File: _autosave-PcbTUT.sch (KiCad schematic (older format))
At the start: 14 parts, among them SW1 SW_Push, U1 ATmega32U4-AU, Y1 16Mhz

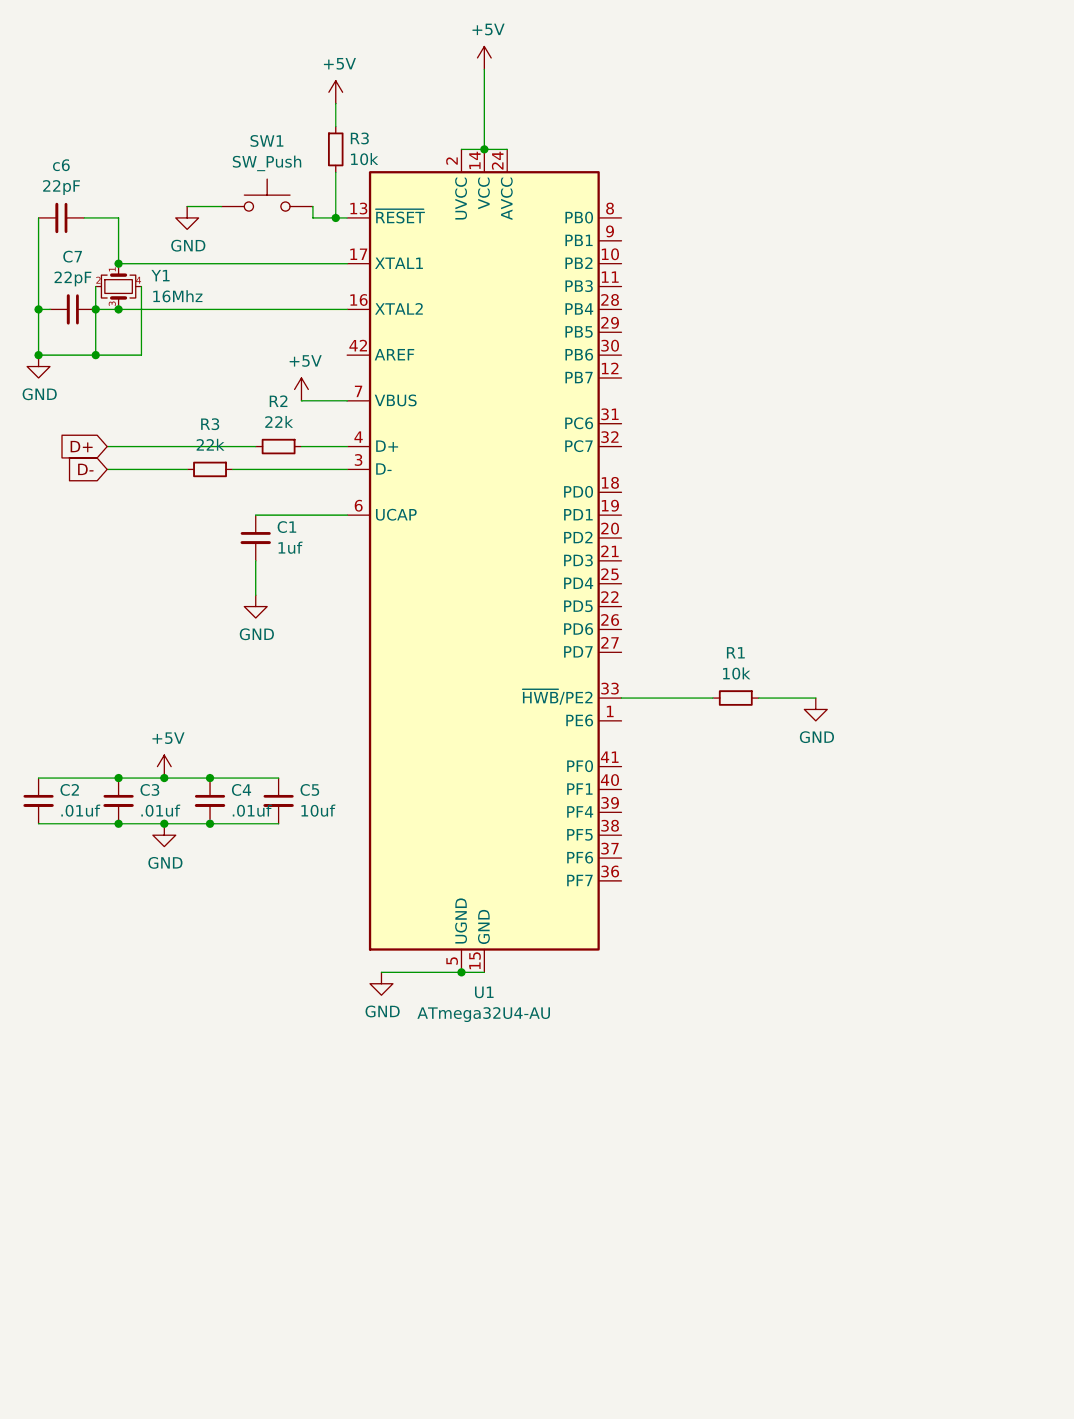
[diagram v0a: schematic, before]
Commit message: up to step 7
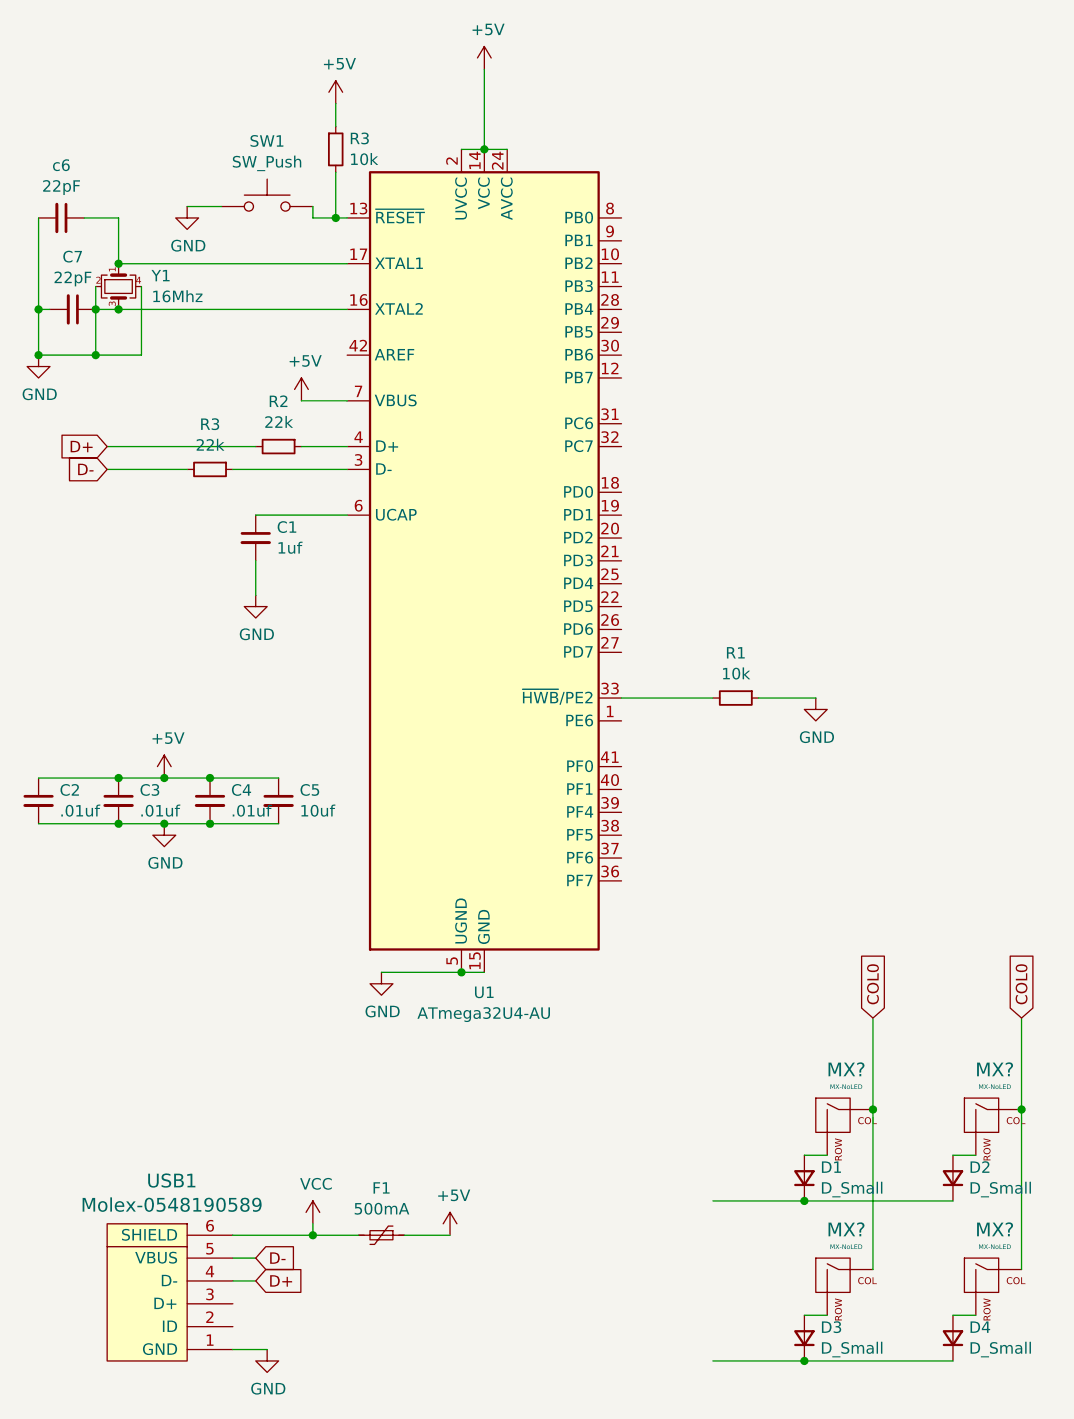
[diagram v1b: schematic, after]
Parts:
- added D1, D2, D3, D4: D_Small, symbol Device:D_Small
- added F1: 500mA, symbol Device:Polyfuse_Small
- added MX? (x4): MX-NoLED, symbol MX_Alps_Hybrid:MX-NoLED
- added USB1: Molex-0548190589, symbol random-keyboard-parts:Molex-0548190589
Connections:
- net labels added: COL0, VCC
- wire segments 41 -> 60
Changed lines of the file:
@@
 Text GLabel 850  2800 0    50   Input ~ 0
 D-
+$Comp
+L random-keyboard-parts:Molex-0548190589 USB1
+U 1 1 5EFB8536
+P 1100 6450
+F 0 "USB1" V 1637 6417 60  0000 C CNN
+F 1 "Molex-0548190589" V 1531 6417 60  0000 C CNN
+F 2 "" H 1100 6450 60  0001 C CNN
+F 3 "" H 1100 6450 60  0001 C CNN
+	1    1100 6450
+	0    -1   -1   0
+$EndComp
+$Comp
+L power:GND #PWR?
+U 1 1 5EFBB31B
+P 1550 6650
+F 0 "#PWR?" H 1550 6400 50  0001 C CNN
+F 1 "GND" H 1555 6477 50  0000 C CNN
+F 2 "" H 1550 6650 50  0001 C CNN
+F 3 "" H 1550 6650 50  0001 C CNN
+	1    1550 6650
+	1    0    0    -1
+$EndComp
+Wire Wire Line
+	1400 6650 1550 6650
+$Comp
+L power:+5V #PWR?
+U 1 1 5EFBCC7A
+P 2350 6150
+F 0 "#PWR?" H 2350 6000 50  0001 C CNN
+F 1 "+5V" H 2365 6323 50  0000 C CNN
+F 2 "" H 2350 6150 50  0001 C CNN
+F 3 "" H 2350 6150 50  0001 C CNN
+	1    2350 6150
+	1    0    0    -1
+$EndComp
+$Comp
+L Device:Polyfuse_Small F1
+U 1 1 5EFBDF67
+P 2050 6150
+F 0 "F1" V 1845 6150 50  0000 C CNN
+F 1 "500mA" V 1936 6150 50  0000 C CNN
+F 2 "" H 2100 5950 50  0001 L CNN
+F 3 "~" H 2050 6150 50  0001 C CNN
+	1    2050 6150
+	0    1    1    0
+$EndComp
+$Comp
+L power:VCC #PWR?
+U 1 1 5EFC0E39
+P 1750 6100
+F 0 "#PWR?" H 1750 5950 50  0001 C CNN
+F 1 "VCC" H 1765 6273 50  0000 C CNN
+F 2 "" H 1750 6100 50  0001 C CNN
+F 3 "" H 1750 6100 50  0001 C CNN
+	1    1750 6100
+	1    0    0    -1
+$EndComp
+Wire Wire Line
+	1950 6150 1750 6150
+Wire Wire Line
+	1750 6100 1750 6150
+Connection ~ 1750 6150
+Wire Wire Line
+	1750 6150 1400 6150
+Wire Wire Line
+	2150 6150 2350 6150
+Text GLabel 1500 6250 2    50   Input ~ 0
+D-
+Text GLabel 1500 6350 2    50   Input ~ 0
+D+
+Wire Wire Line
+	1500 6350 1400 6350
+Wire Wire Line
+	1400 6250 1500 6250
+$Comp
+L MX_Alps_Hybrid:MX-NoLED MX?
+U 1 1 5EFC6D22
+P 4050 5650
+F 0 "MX?" H 4083 5873 60  0000 C CNN
+F 1 "MX-NoLED" H 4083 5799 20  0000 C CNN
+F 2 "" H 3425 5625 60  0001 C CNN
+F 3 "" H 3425 5625 60  0001 C CNN
+	1    4050 5650
+	1    0    0    -1
+$EndComp
+$Comp
+L Device:D_Small D1
+U 1 1 5EFC81BE
+P 3900 5900
+F 0 "D1" V 3946 5830 50  0000 R CNN
+F 1 "D_Small" V 3855 5830 50  0000 R CNN
+F 2 "" V 3900 5900 50  0001 C CNN
+F 3 "~" V 3900 5900 50  0001 C CNN
+	1    3900 5900
+	0    -1   -1   0
+$EndComp
+Wire Wire Line
+	4000 5800 3900 5800
+$Comp
+L MX_Alps_Hybrid:MX-NoLED MX?
+U 1 1 5EFC9D6F
+P 4700 5650
+F 0 "MX?" H 4733 5873 60  0000 C CNN
+F 1 "MX-NoLED" H 4733 5799 20  0000 C CNN
+F 2 "" H 4075 5625 60  0001 C CNN
+F 3 "" H 4075 5625 60  0001 C CNN
+	1    4700 5650
+	1    0    0    -1
+$EndComp
+$Comp
+L MX_Alps_Hybrid:MX-NoLED MX?
+U 1 1 5EFCA473
+P 4700 6350
+F 0 "MX?" H 4733 6573 60  0000 C CNN
+F 1 "MX-NoLED" H 4733 6499 20  0000 C CNN
+F 2 "" H 4075 6325 60  0001 C CNN
+F 3 "" H 4075 6325 60  0001 C CNN
+	1    4700 6350
+	1    0    0    -1
+$EndComp
+$Comp
+L MX_Alps_Hybrid:MX-NoLED MX?
+U 1 1 5EFCADDE
+P 4050 6350
+F 0 "MX?" H 4083 6573 60  0000 C CNN
+F 1 "MX-NoLED" H 4083 6499 20  0000 C CNN
+F 2 "" H 3425 6325 60  0001 C CNN
+F 3 "" H 3425 6325 60  0001 C CNN
+	1    4050 6350
+	1    0    0    -1
+$EndComp
+$Comp
+L Device:D_Small D2
+U 1 1 5EFCB34D
+P 4550 5900
+F 0 "D2" V 4596 5830 50  0000 R CNN
+F 1 "D_Small" V 4505 5830 50  0000 R CNN
+F 2 "" V 4550 5900 50  0001 C CNN
+F 3 "~" V 4550 5900 50  0001 C CNN
+	1    4550 5900
+	0    -1   -1   0
+$EndComp
+$Comp
+L Device:D_Small D4
+U 1 1 5EFCBBCD
+P 4550 6600
+F 0 "D4" V 4596 6530 50  0000 R CNN
+F 1 "D_Small" V 4505 6530 50  0000 R CNN
+F 2 "" V 4550 6600 50  0001 C CNN
+F 3 "~" V 4550 6600 50  0001 C CNN
+	1    4550 6600
+	0    -1   -1   0
+$EndComp
+$Comp
+L Device:D_Small D3
+U 1 1 5EFCC218
+P 3900 6600
+F 0 "D3" V 3946 6530 50  0000 R CNN
+F 1 "D_Small" V 3855 6530 50  0000 R CNN
+F 2 "" V 3900 6600 50  0001 C CNN
+F 3 "~" V 3900 6600 50  0001 C CNN
+	1    3900 6600
+	0    -1   -1   0
+$EndComp
+Wire Wire Line
+	3900 6500 4000 6500
+Wire Wire Line
+	4550 6500 4650 6500
+Wire Wire Line
+	4550 5800 4650 5800
+Wire Wire Line
+	4200 6300 4200 5600
+Connection ~ 4200 5600
+Wire Wire Line
+	4200 5600 4200 5200
+Wire Wire Line
+	4850 6300 4850 5600
+Connection ~ 4850 5600
+Wire Wire Line
+	4850 5600 4850 5200
+Wire Wire Line
+	4550 6700 3900 6700
+Connection ~ 3900 6700
+Wire Wire Line
+	3900 6700 3500 6700
+Wire Wire Line
+	4550 6000 3900 6000
+Connection ~ 3900 6000
+Wire Wire Line
+	3900 6000 3500 6000
+Text GLabel 4200 5200 1    50   Input ~ 0
+COL0
+Text GLabel 4850 5200 1    50   Input ~ 0
+COL0
 $EndSCHEMATC
